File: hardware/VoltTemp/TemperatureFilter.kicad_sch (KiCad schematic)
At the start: 9 parts, among them U4 TLV9062xD

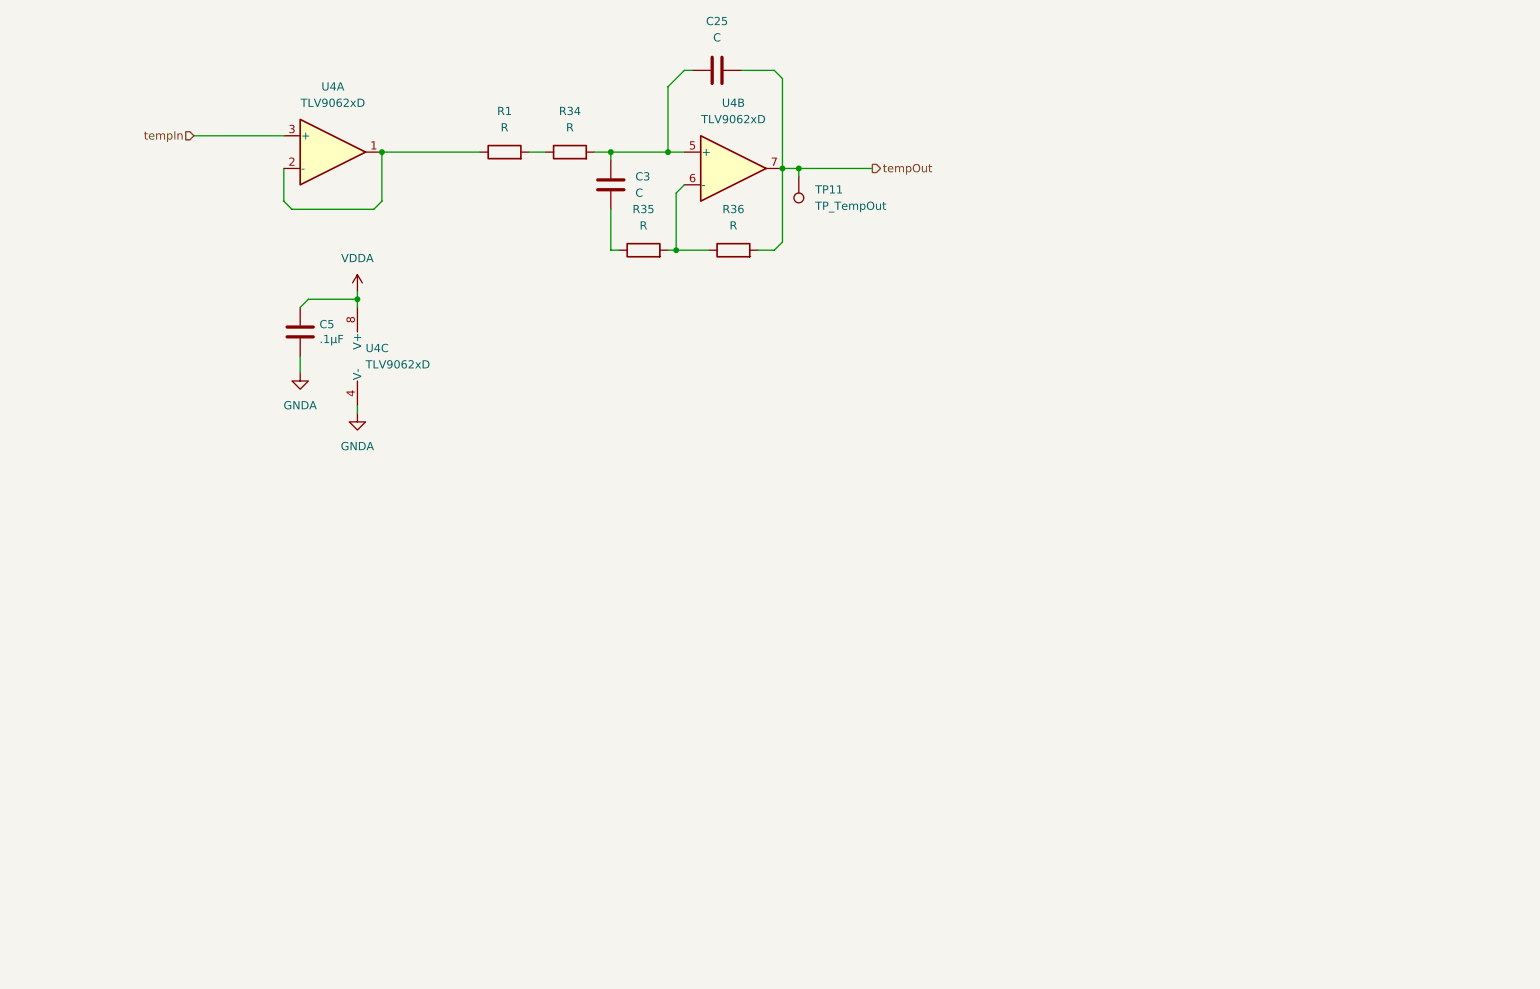
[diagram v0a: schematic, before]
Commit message: most layout done
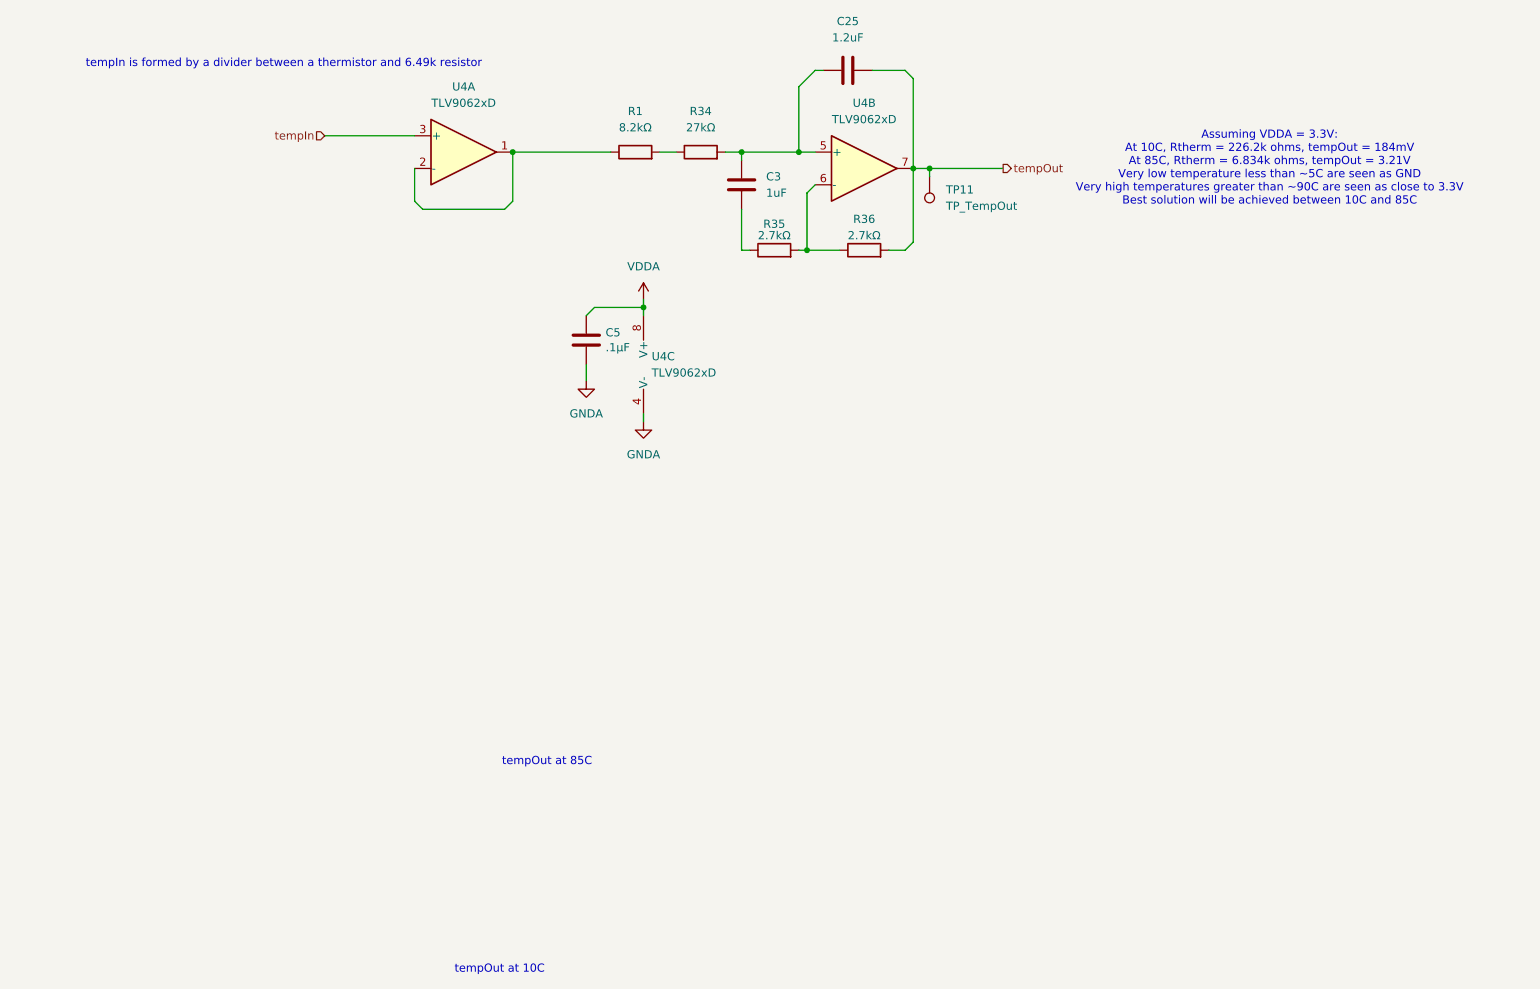
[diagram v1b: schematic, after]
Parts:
- C25: value C -> 1.2uF
- C3: value C -> 1uF; P/N (none) -> MLASU168SB5105KTNA01
- R1: value R -> 8.2kΩ
- R34: value R -> 27kΩ
- R35, R36: value R -> 2.7kΩ
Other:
- note added: "Assuming VDDA = 3.3V: At 10C, Rtherm = 226.2k ohms, tempOut = 184mV At 85C, Rtherm = 6.834k ohms, tempOut = 3.21V Very low temperature less than ~5C are seen as GND Very high temperatures greater than ~90C are seen as close to 3.3V Best solution will be achieved between 10C and 85C"
- note added: "tempIn is formed by a divider between a thermistor and 6.49k resistor"
- note added: "tempOut at 10C"
- note added: "tempOut at 85C"
- moved on the sheet: C25, C3, C5, R1, R34, R35, R36, TP11, U4A, U4B, U4C
